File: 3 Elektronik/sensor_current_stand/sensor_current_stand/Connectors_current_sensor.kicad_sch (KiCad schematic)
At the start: 4 parts, among them J3 DC37_Plug_MountingHoles, J4 DC37_Plug_MountingHoles, J5 DC37_Plug_MountingHoles, J6 DC37_Plug_MountingHoles

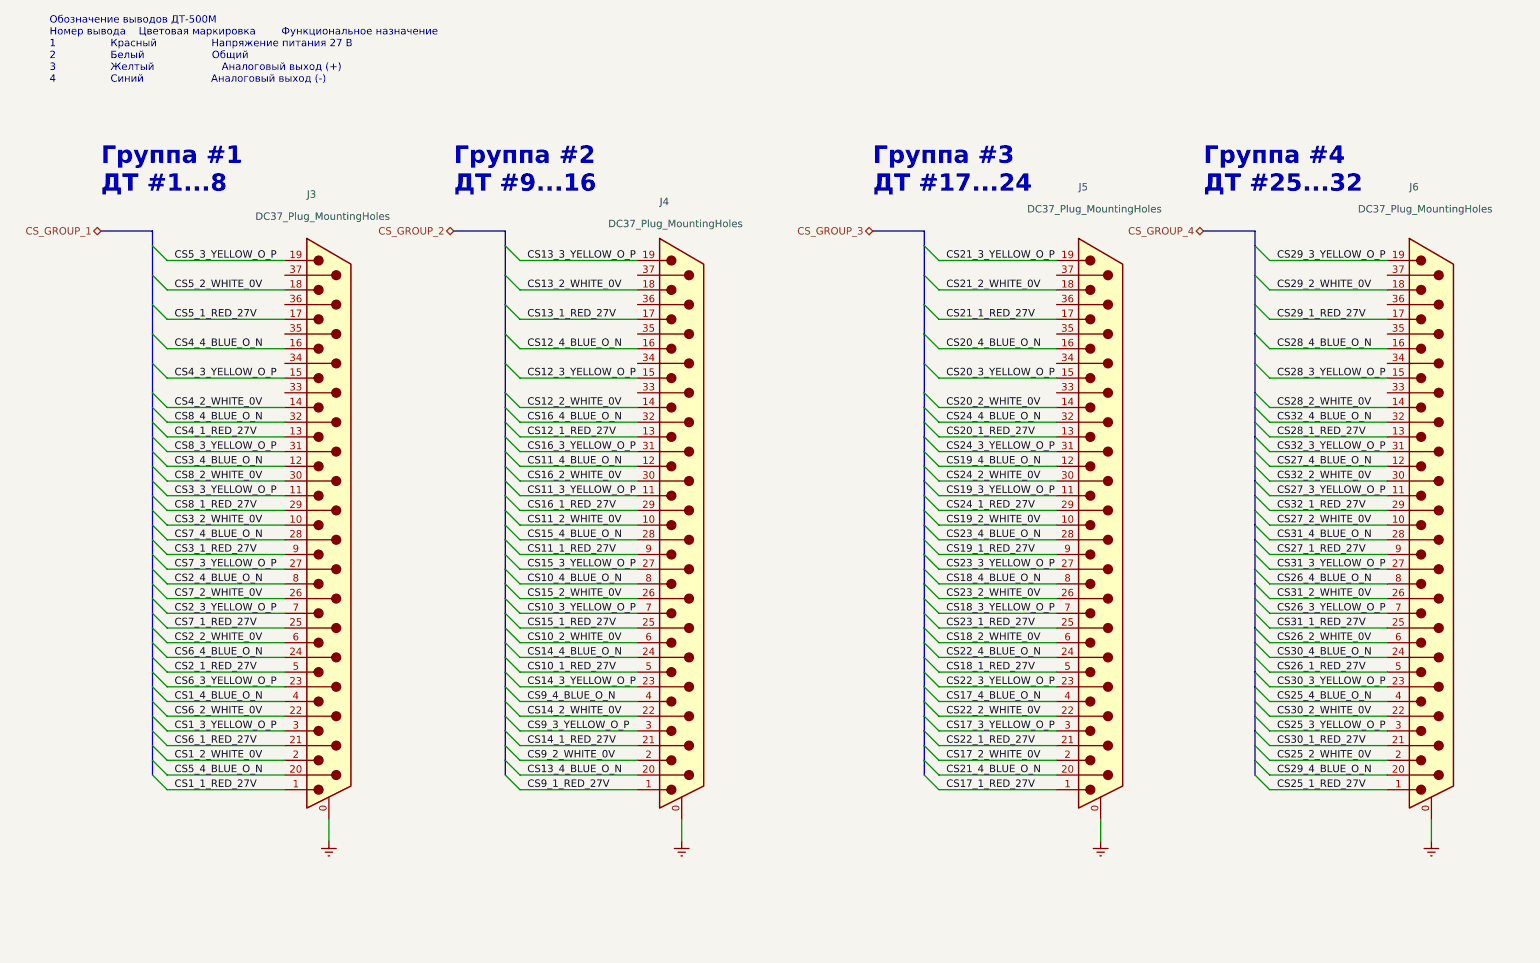
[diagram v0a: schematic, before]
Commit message: разработка
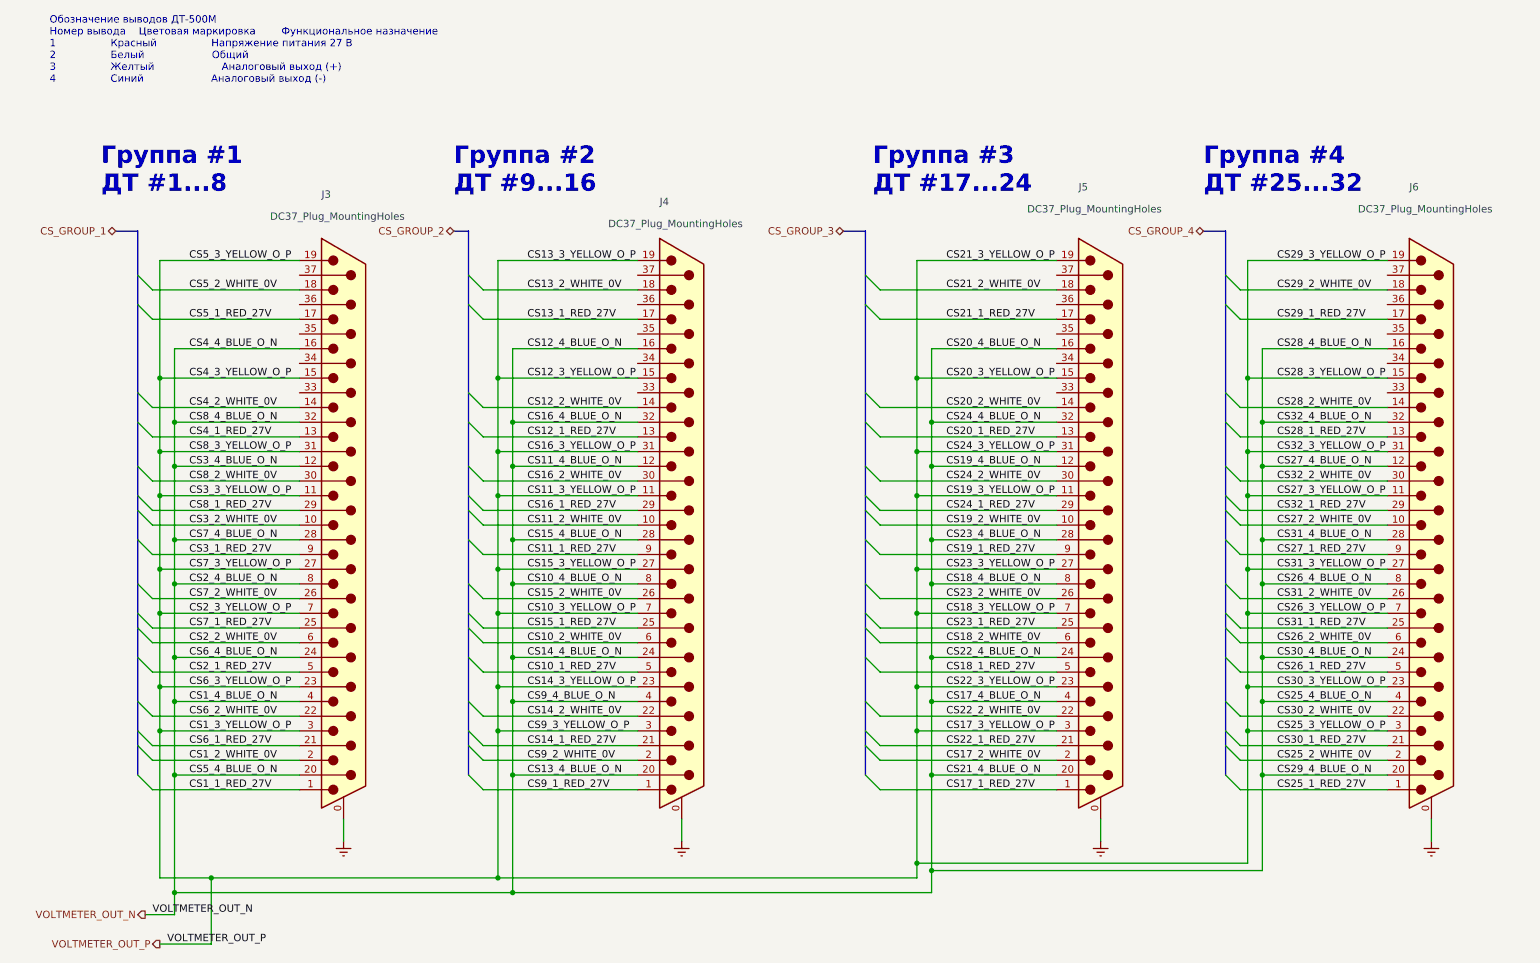
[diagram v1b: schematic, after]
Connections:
- net CS11_3_YELLOW_O_P is gone; now on net VOLTMETER_OUT_P: J4.11
- net CS11_4_BLUE_O_N is gone; now on net VOLTMETER_OUT_N: J4.12
- net CS12_3_YELLOW_O_P is gone; now on net VOLTMETER_OUT_P: J4.15
- net CS12_4_BLUE_O_N is gone; now on net VOLTMETER_OUT_N: J4.16
- net CS13_3_YELLOW_O_P is gone; now on net VOLTMETER_OUT_P: J4.19
- net CS13_4_BLUE_O_N is gone; now on net VOLTMETER_OUT_N: J4.20
- net CS14_3_YELLOW_O_P is gone; now on net VOLTMETER_OUT_P: J4.23
- net CS14_4_BLUE_O_N is gone; now on net VOLTMETER_OUT_N: J4.24
- net CS15_3_YELLOW_O_P is gone; now on net VOLTMETER_OUT_P: J4.27
- net CS15_4_BLUE_O_N is gone; now on net VOLTMETER_OUT_N: J4.28
- net CS16_3_YELLOW_O_P is gone; now on net VOLTMETER_OUT_P: J4.31
- net CS16_4_BLUE_O_N is gone; now on net VOLTMETER_OUT_N: J4.32
- net CS17_3_YELLOW_O_P is gone; now on net VOLTMETER_OUT_P: J5.3
- net CS17_4_BLUE_O_N is gone; now on net VOLTMETER_OUT_N: J5.4
- net CS18_3_YELLOW_O_P is gone; now on net VOLTMETER_OUT_P: J5.7
- net CS18_4_BLUE_O_N is gone; now on net VOLTMETER_OUT_N: J5.8
- net CS19_3_YELLOW_O_P is gone; now on net VOLTMETER_OUT_P: J5.11
- net CS19_4_BLUE_O_N is gone; now on net VOLTMETER_OUT_N: J5.12
- net CS1_3_YELLOW_O_P is gone; now on net VOLTMETER_OUT_P: J3.3
- net CS1_4_BLUE_O_N is gone; now on net VOLTMETER_OUT_N: J3.4
- net CS20_3_YELLOW_O_P is gone; now on net VOLTMETER_OUT_P: J5.15
- net CS20_4_BLUE_O_N is gone; now on net VOLTMETER_OUT_N: J5.16
- net CS21_3_YELLOW_O_P is gone; now on net VOLTMETER_OUT_P: J5.19
- net CS21_4_BLUE_O_N is gone; now on net VOLTMETER_OUT_N: J5.20
- net CS22_3_YELLOW_O_P is gone; now on net VOLTMETER_OUT_P: J5.23
- net CS22_4_BLUE_O_N is gone; now on net VOLTMETER_OUT_N: J5.24
- net CS23_3_YELLOW_O_P is gone; now on net VOLTMETER_OUT_P: J5.27
- net CS23_4_BLUE_O_N is gone; now on net VOLTMETER_OUT_N: J5.28
- net CS24_3_YELLOW_O_P is gone; now on net VOLTMETER_OUT_P: J5.31
- net CS24_4_BLUE_O_N is gone; now on net VOLTMETER_OUT_N: J5.32
- net CS25_3_YELLOW_O_P is gone; now on net VOLTMETER_OUT_P: J6.3
- net CS25_4_BLUE_O_N is gone; now on net VOLTMETER_OUT_N: J6.4
- net CS26_3_YELLOW_O_P is gone; now on net VOLTMETER_OUT_P: J6.7
- net CS26_4_BLUE_O_N is gone; now on net VOLTMETER_OUT_N: J6.8
- net CS27_3_YELLOW_O_P is gone; now on net VOLTMETER_OUT_P: J6.11
- net CS27_4_BLUE_O_N is gone; now on net VOLTMETER_OUT_N: J6.12
- net CS28_3_YELLOW_O_P is gone; now on net VOLTMETER_OUT_P: J6.15
- net CS28_4_BLUE_O_N is gone; now on net VOLTMETER_OUT_N: J6.16
- net CS29_3_YELLOW_O_P is gone; now on net VOLTMETER_OUT_P: J6.19
- net CS29_4_BLUE_O_N is gone; now on net VOLTMETER_OUT_N: J6.20
- net CS2_3_YELLOW_O_P is gone; now on net VOLTMETER_OUT_P: J3.7
- net CS2_4_BLUE_O_N is gone; now on net VOLTMETER_OUT_N: J3.8
- net CS30_3_YELLOW_O_P is gone; now on net VOLTMETER_OUT_P: J6.23
- net CS30_4_BLUE_O_N is gone; now on net VOLTMETER_OUT_N: J6.24
- net CS31_3_YELLOW_O_P is gone; now on net VOLTMETER_OUT_P: J6.27
- net CS31_4_BLUE_O_N is gone; now on net VOLTMETER_OUT_N: J6.28
- net CS32_3_YELLOW_O_P is gone; now on net VOLTMETER_OUT_P: J6.31
- net CS32_4_BLUE_O_N is gone; now on net VOLTMETER_OUT_N: J6.32
- net CS3_3_YELLOW_O_P is gone; now on net VOLTMETER_OUT_P: J3.11
- net CS3_4_BLUE_O_N is gone; now on net VOLTMETER_OUT_N: J3.12
- net CS4_3_YELLOW_O_P is gone; now on net VOLTMETER_OUT_P: J3.15
- net CS4_4_BLUE_O_N is gone; now on net VOLTMETER_OUT_N: J3.16
- net CS5_3_YELLOW_O_P is gone; now on net VOLTMETER_OUT_P: J3.19
- net CS5_4_BLUE_O_N is gone; now on net VOLTMETER_OUT_N: J3.20
- net CS6_3_YELLOW_O_P is gone; now on net VOLTMETER_OUT_P: J3.23
- net CS6_4_BLUE_O_N is gone; now on net VOLTMETER_OUT_N: J3.24
- net CS7_3_YELLOW_O_P is gone; now on net VOLTMETER_OUT_P: J3.27
- net CS7_4_BLUE_O_N is gone; now on net VOLTMETER_OUT_N: J3.28
- net CS8_3_YELLOW_O_P is gone; now on net VOLTMETER_OUT_P: J3.31
- net CS8_4_BLUE_O_N is gone; now on net VOLTMETER_OUT_N: J3.32
- net CS9_3_YELLOW_O_P is gone; now on net VOLTMETER_OUT_P: J4.3
- net CS9_4_BLUE_O_N is gone; now on net VOLTMETER_OUT_N: J4.4
- net CS10_3_YELLOW_O_P renamed VOLTMETER_OUT_P
- net CS10_4_BLUE_O_N renamed VOLTMETER_OUT_N
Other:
- moved on the sheet: J3

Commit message: Группа 1 разведена но не проверена
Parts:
- removed J3, J4, J5, J6: DC37_Plug_MountingHoles, Connector_Dsub:DSUB-37_Male_Vertical_P2.77x2.84mm_MountingHoles, symbol Connector:DC37_Plug_MountingHoles
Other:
- note removed: "Группа #1 ДТ #1...8"
- note removed: "Группа #2 ДТ #9...16"
- note removed: "Группа #3 ДТ #17...24"
- note removed: "Группа #4 ДТ #25...32"
- note removed: "Обозначение выводов ДТ-500М Номер вывода Цветовая маркировка Функциональное назначение 1 Красный Напряжение питания 27 В 2 Белый Общий 3 Желтый Аналоговый выход (+) 4 Синий Аналоговый выход (-)"
